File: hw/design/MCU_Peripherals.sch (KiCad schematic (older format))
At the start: 1 part

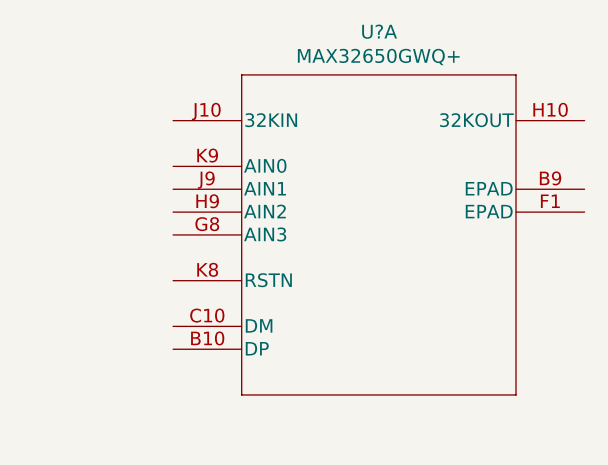
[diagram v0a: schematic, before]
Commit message: Slow day for the project, wasn't really feeling inspired.
Actually quite tilted that 0 keypad switch manufacturers offer schematic
symbols and footprints of their products.

Oh well, added uUSB traces and moves the sheets around to prepare for PMU
integration.

It's also painfully obvious that there's a lot to do for parts I have already
traced; I need to make sure current, voltage, etc. are all in line with specs
for every piece. Kinda feels like I have made big strides already, but I am not
ready to stop.
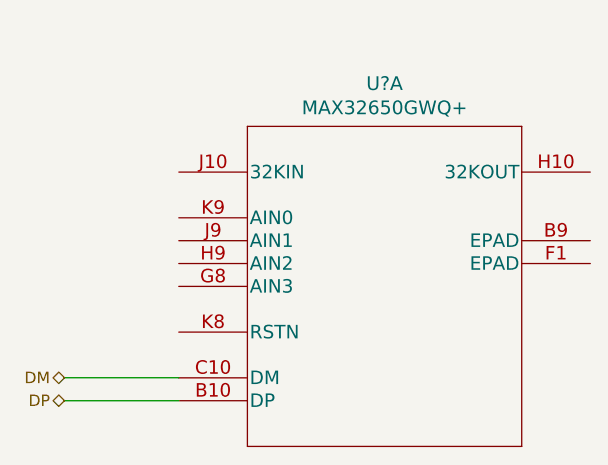
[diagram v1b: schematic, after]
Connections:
- net DP: now reaches U?.B10 (DP)
- net DM: now reaches U?.C10 (DM)
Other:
- moved on the sheet: U?A
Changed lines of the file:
@@
 $Descr A4 11693 8268
 encoding utf-8
-Sheet 5 7
+Sheet 4 7
 Title ""
 Date ""
@@
 L MAX32650GWP:MAX32650GWQ+ U?
 U 1 1 5E17F23E
-P 4975 3625
-F 0 "U?" H 5875 4012 60  0000 C CNN
-F 1 "MAX32650GWQ+" H 5875 3906 60  0000 C CNN
-F 2 "21-100240A_W964A4+1" H 5875 3865 60  0001 C CNN
-F 3 "" H 4975 3625 60  0000 C CNN
-	1    4975 3625
+P 5000 3850
+F 0 "U?" H 5900 4237 60  0000 C CNN
+F 1 "MAX32650GWQ+" H 5900 4131 60  0000 C CNN
+F 2 "21-100240A_W964A4+1" H 5900 4090 60  0001 C CNN
+F 3 "" H 5000 3850 60  0000 C CNN
+	1    5000 3850
 	1    0    0    -1
 $EndComp
+Wire Wire Line
+	5000 4750 4500 4750
+Wire Wire Line
+	5000 4850 4500 4850
+Text HLabel 4500 4750 0    50   BiDi ~ 0
+DM
+Text HLabel 4500 4850 0    50   BiDi ~ 0
+DP
 $EndSCHEMATC
